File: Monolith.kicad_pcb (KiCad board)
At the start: 2 copper layers, 89.9 x 42.7 mm, 82 parts, among them J1 USB_B_Micro, J2 Conn_01x11, J3 Conn_01x11, J4 Conn_01x02, J5 Conn_01x02, J7 Conn_01x08, Q1 BC818, Q2 BC818, U1 ADS1299IPAGR, U12 ESP32-S3-MINI-1, U2 AMS1117-3.3, U3 CP2102N-A02-GQFN28R, U4 LM2664M6, U5 TLV70025QDDCRQ1, U6 TPS72325

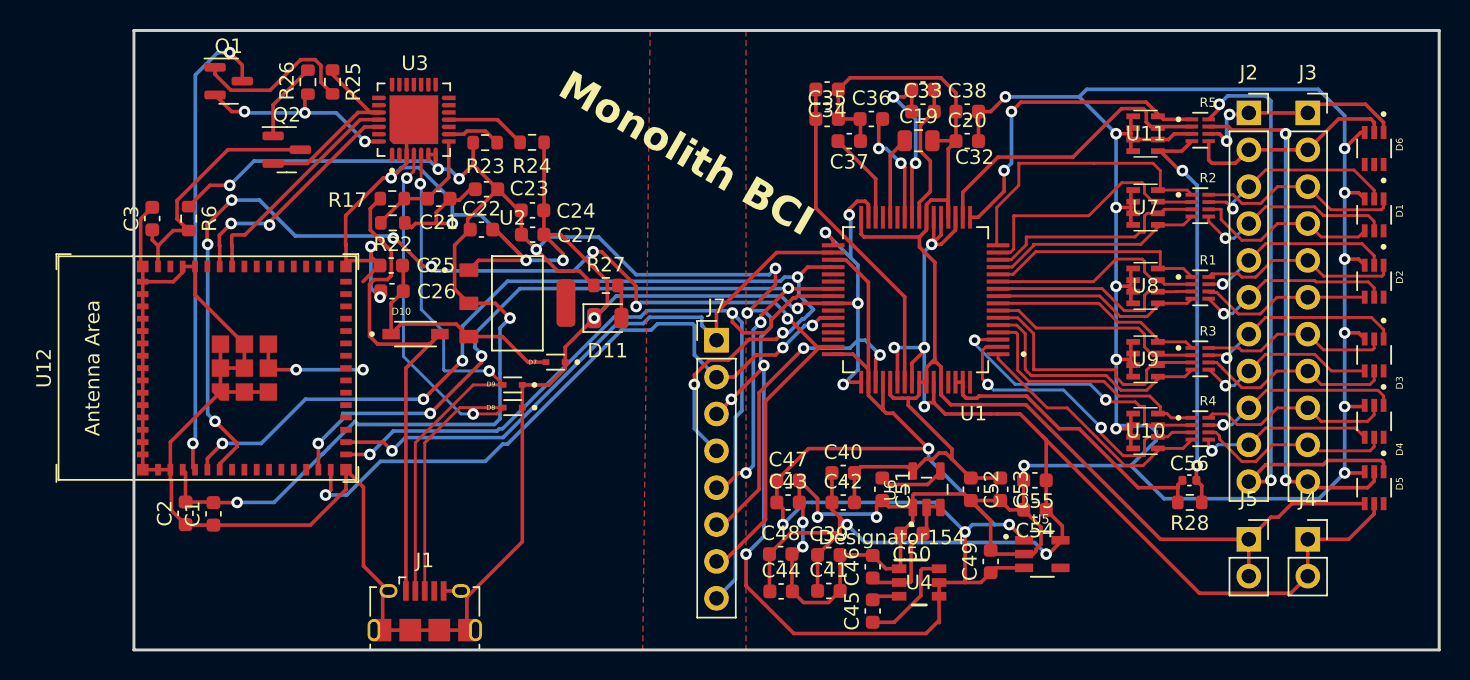
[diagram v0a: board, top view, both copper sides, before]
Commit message: fixes
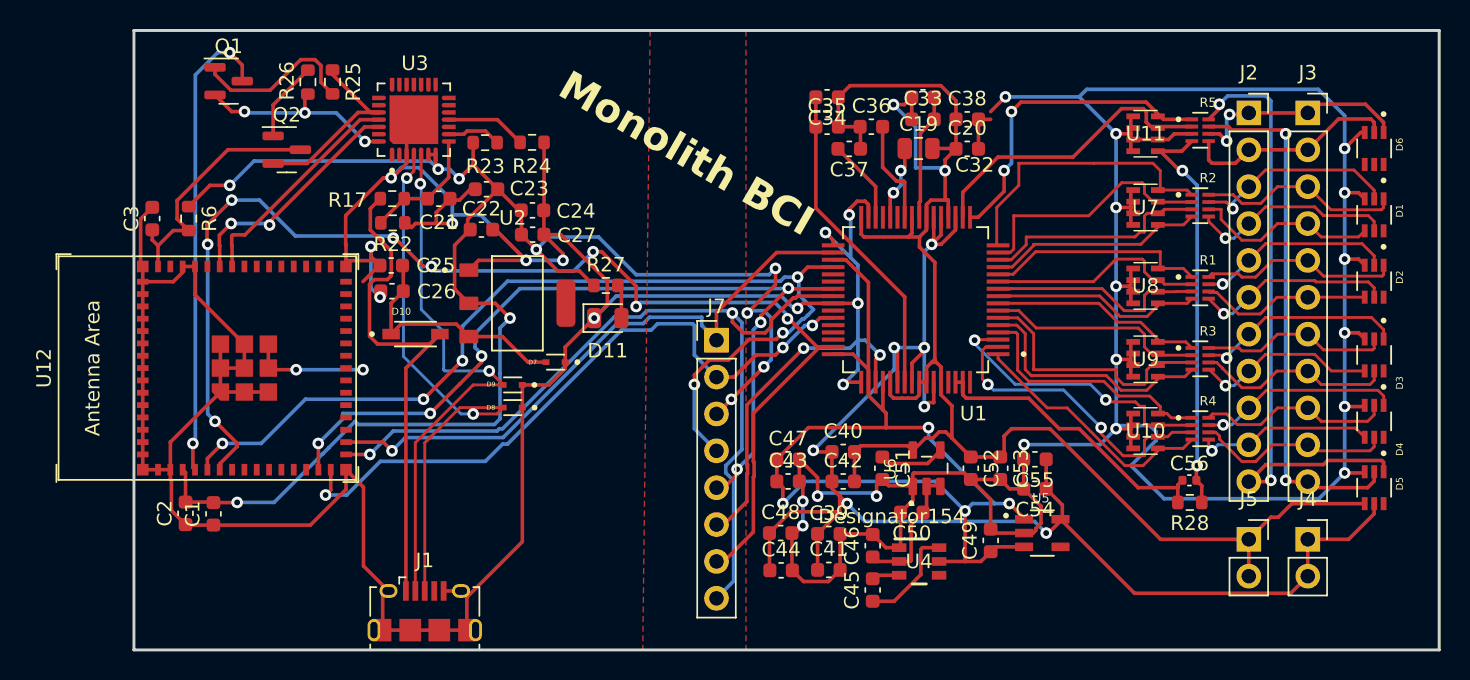
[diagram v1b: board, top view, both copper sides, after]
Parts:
- C20: value 1uF -> 0.1uF
- moved C40 1.45 mm to (227.7, 150.4)
- moved C41 1.45 mm to (226.7, 158.6)
- moved C42 1.45 mm to (227.7, 152.5)
- moved C43 1.45 mm to (223.9, 152.5)
- moved C44 1.45 mm to (223.4, 158.6)
- moved C45 1.45 mm to (229.7, 160.0)
- moved C46 1.45 mm to (229.7, 156.9)
- moved C47 1.45 mm to (223.9, 151.0)
- moved C49 1.45 mm to (237.8, 156.5)
- moved C55 1.45 mm to (240.9, 151.0)
- moved U4 1.45 mm to (232.9, 158.0)
- moved C39 1.45 mm to (226.7, 156.1)
- moved C48 1.45 mm to (223.4, 156.0)
- moved C50 1.45 mm to (232.4, 154.6)
- moved C51 1.45 mm to (230.4, 151.6)
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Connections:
- C32 pad 1: Net-(U1-VREFN) -> /AVSS
- C33 pad 1: Net-(U1-VREFN) -> /AVSS
- U1 pad 25: Net-(U1-VREFN) -> /AVSS
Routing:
- net +3V3: track 222.7 -> 185.7 mm, vias 15 -> 14
- net Net-(U1-VREFN): track 12.0 -> 0.00 mm, vias 2 -> 0
- net /AVDD: track 109.6 -> 105.1 mm, vias 6 -> 7
- net /AVSS: track 108.6 -> 112.9 mm, vias 0 -> 2
- net Net-(U1-VREFP): track 9.80 -> 8.70 mm
- net Net-(U1-VCAP4): track 7.92 -> 7.15 mm, vias 2 -> 0
- net GNDA: track 195.4 -> 194.8 mm
- net Net-(U1-VCAP3): track 22.7 -> 22.2 mm
- net Net-(U1-VCAP2): track 6.32 -> 5.79 mm
- net Net-(U1-VCAP1): track 5.69 -> 5.15 mm, vias 0 -> 2
